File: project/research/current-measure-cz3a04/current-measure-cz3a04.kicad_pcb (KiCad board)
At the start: 2 copper layers, 29 x 35.2 mm, 9 parts, among them J1 In, J2 Out, J3 Sensor, U1 CZ-3A04

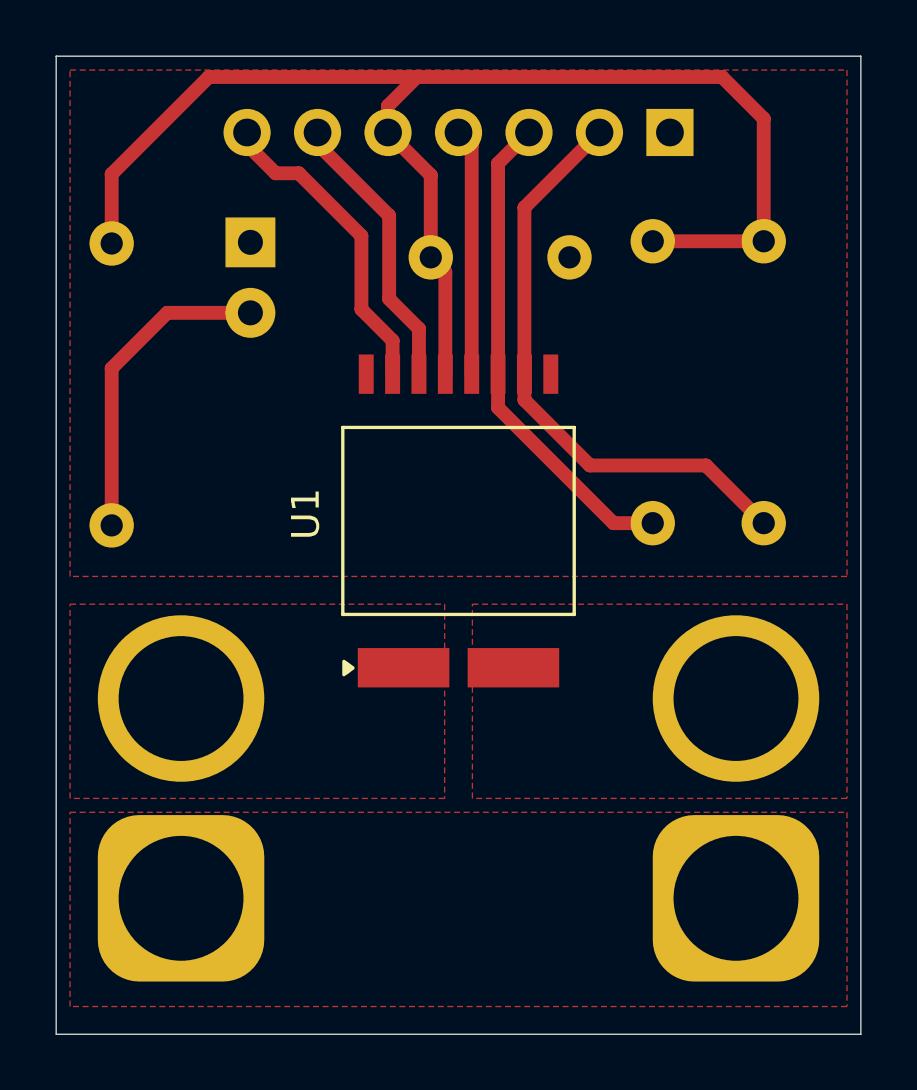
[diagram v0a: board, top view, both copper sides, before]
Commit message: 2026/04/23/17:05
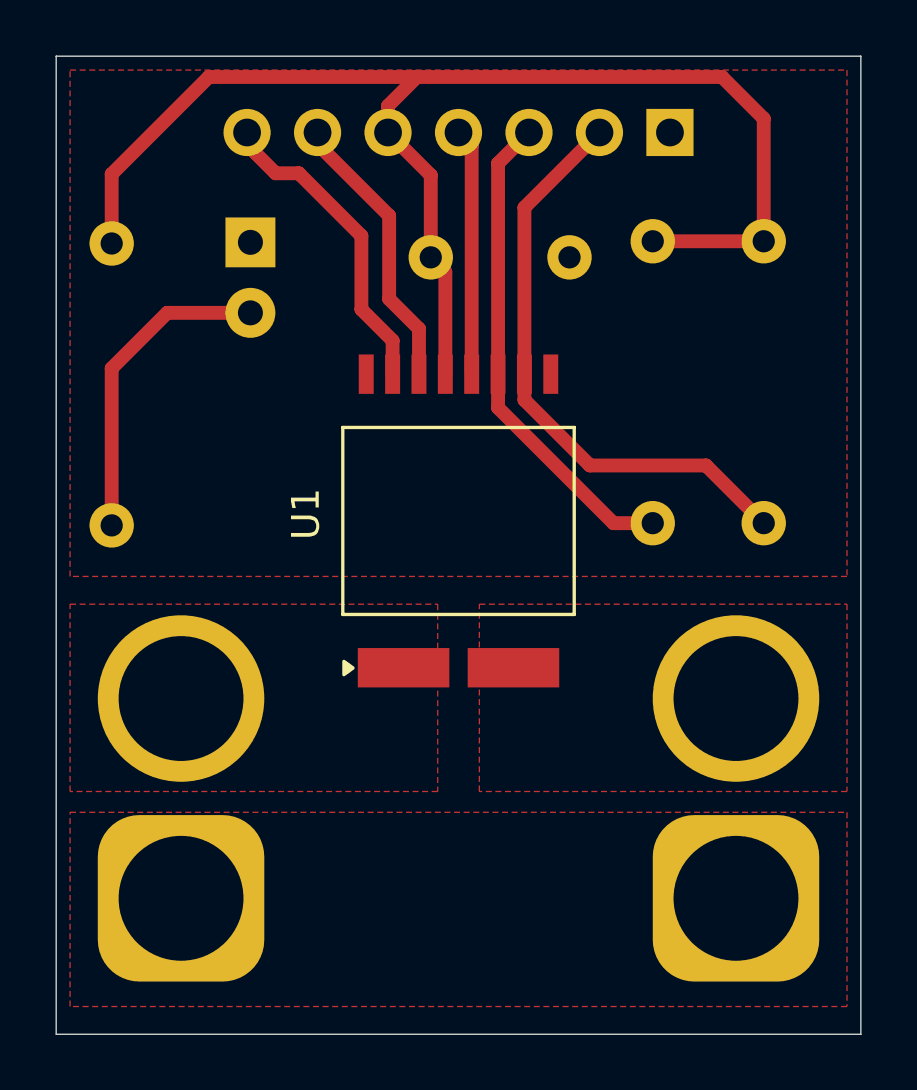
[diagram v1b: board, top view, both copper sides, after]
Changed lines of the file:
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@@
 		(priority 1)
 		(connect_pads yes
-			(clearance 0.5)
+			(clearance 0.75)
 		)
-		(min_thickness 0.25)
+		(min_thickness 0.75)
 		(fill yes
 			(thermal_gap 0.5)
-			(thermal_bridge_width 0.5)
+			(thermal_bridge_width 0.75)
 			(island_removal_mode 0)
 		)
@@
 		(polygon
 			(pts
-				(xy 144 110) (xy 130.5 110) (xy 130.5 103) (xy 144 103)
+				(xy 144 109.75) (xy 130.75 109.75) (xy 130.75 103) (xy 144 103)
 			)
 		)
@@
 		(polygon
 			(pts
-				(xy 116 103) (xy 129.5 103) (xy 129.5 110) (xy 116 110)
+				(xy 116 103) (xy 129.25 103) (xy 129.25 109.75) (xy 116 109.75)
 			)
 		)
